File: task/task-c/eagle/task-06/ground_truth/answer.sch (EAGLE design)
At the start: 12 parts, among them IC1 16F84, U1 78L05

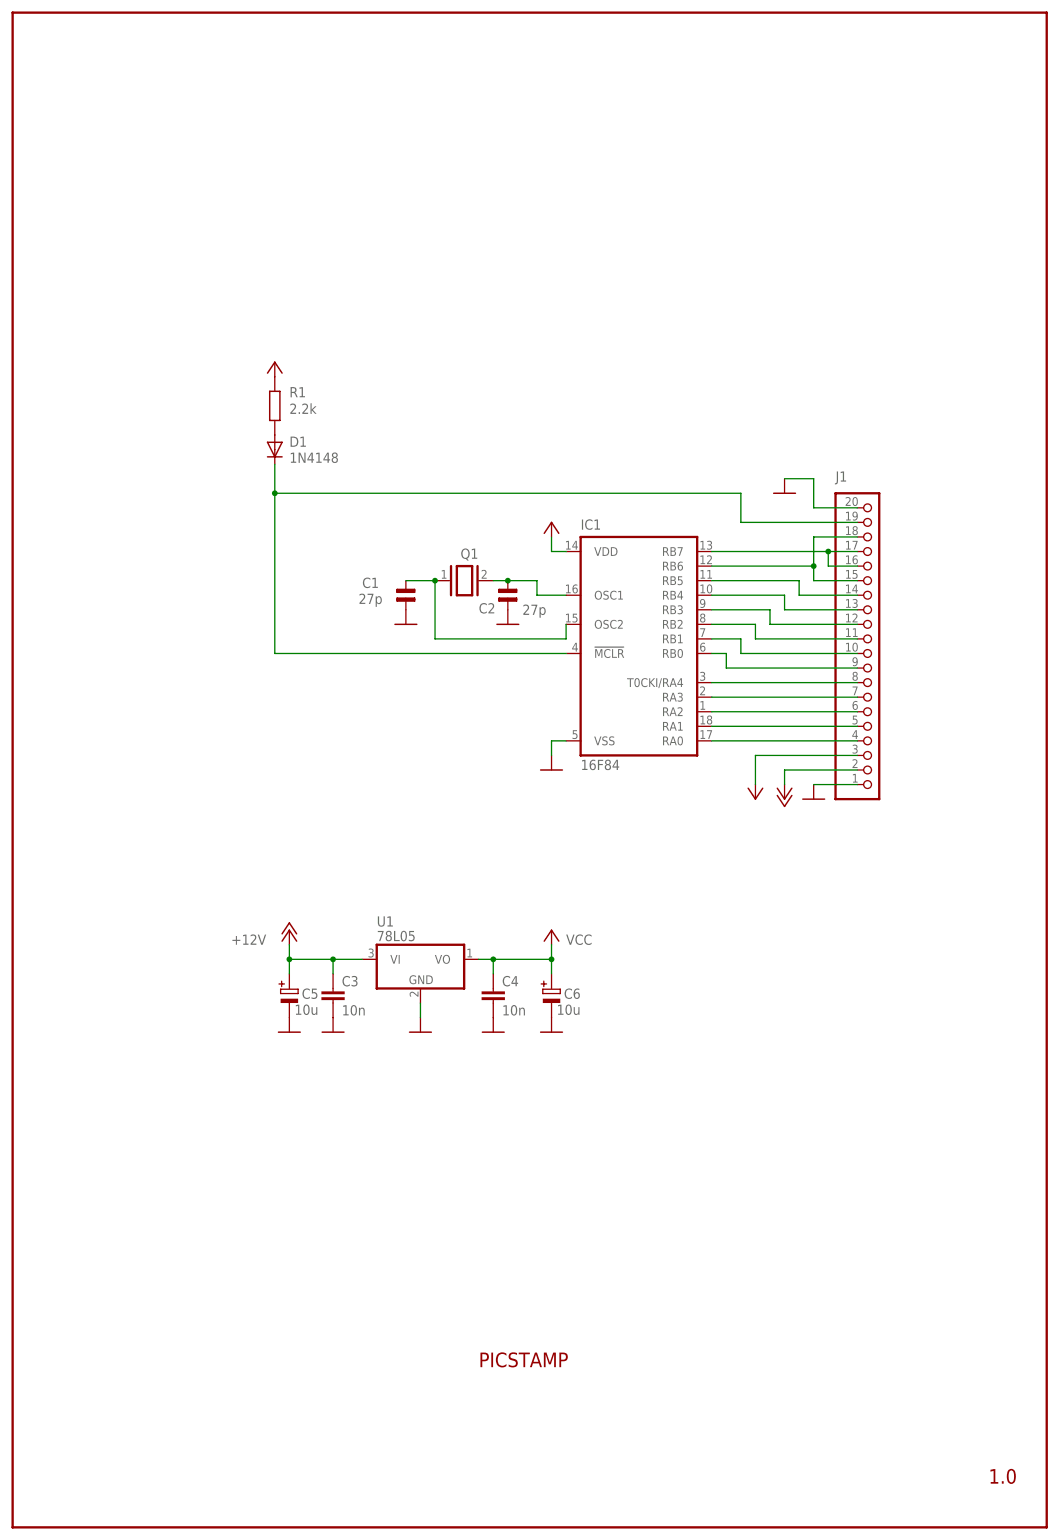
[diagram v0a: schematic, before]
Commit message: Refine engineering task metadata and instructions
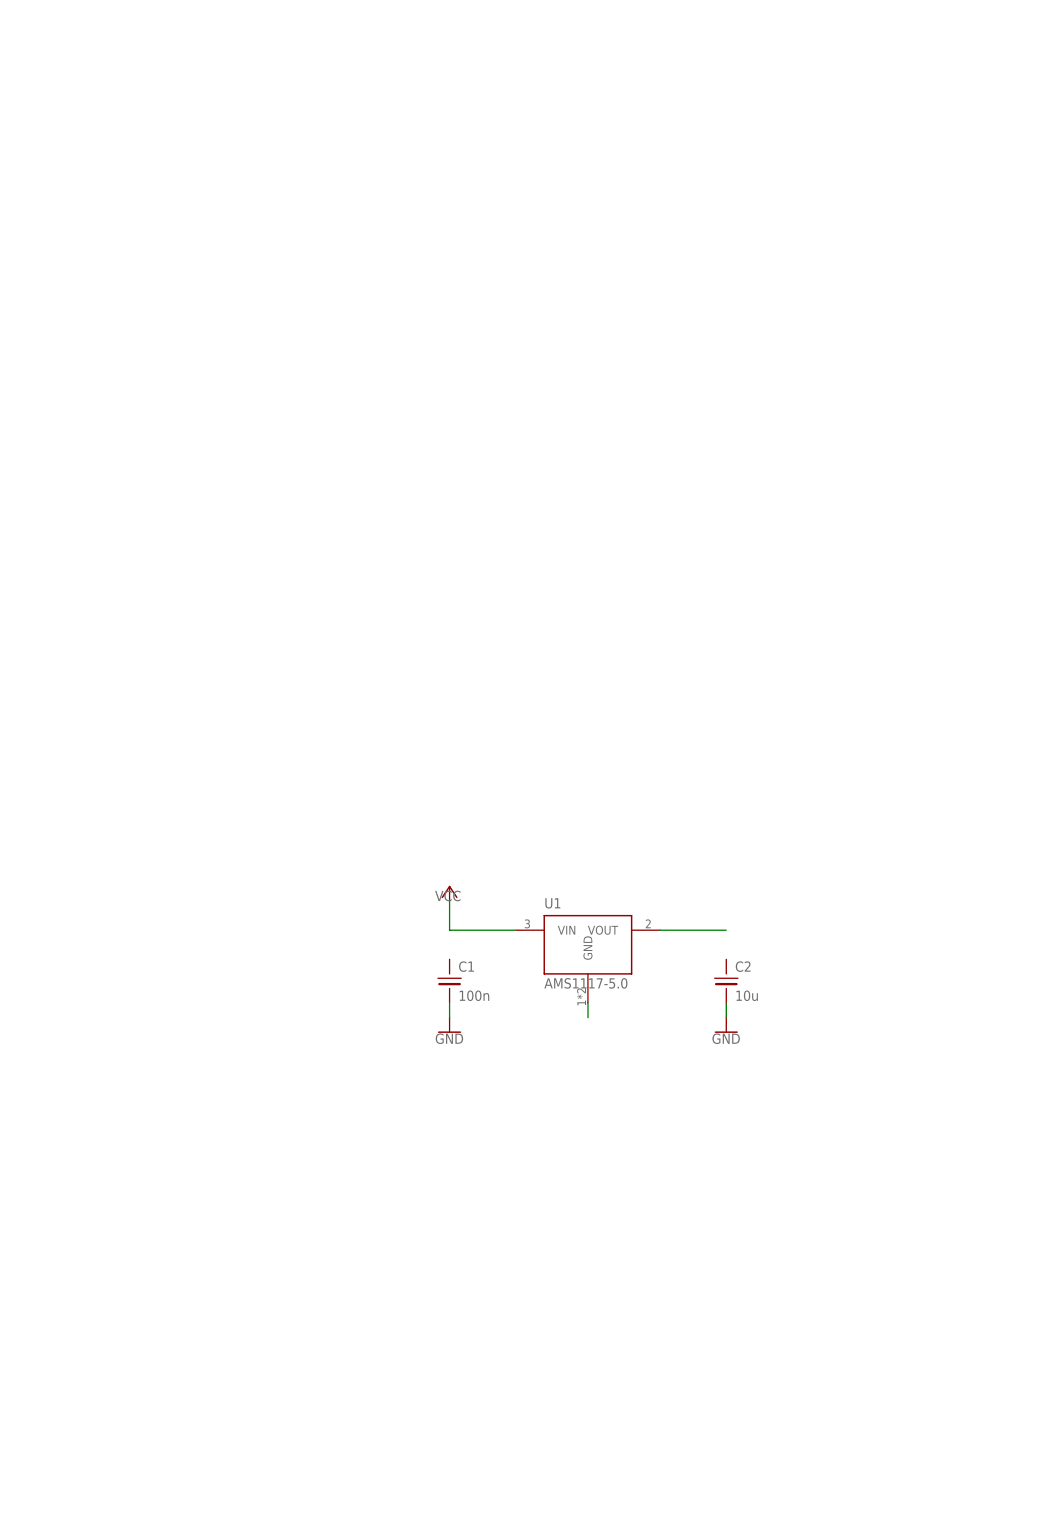
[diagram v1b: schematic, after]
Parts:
- removed C3, C4: 10n, rcl:C-EU025-025X050
- removed C5, C6: 10u, polcap:E2,5-6
- removed D1: 1N4148, diode:1N4148
- removed IC1: 16F84, microchip:PIC16F84AP
- removed J1: (no value), PINHEAD:PINHD-1X20
- removed Q1: (no value), special:XTAL/S
- removed R1: 2.2k, rcl:R-EU_0207/10
- C1: value 27p -> 100n; device capacitor-wima:C2.5/2 -> rcl:C-EU050-025X075
- C2: value 27p -> 10u; device capacitor-wima:C2.5/2 -> rcl:C-EU050-025X075
- U1: value 78L05 -> AMS1117-5.0; device linear:78LXXZ -> v-reg:AMS1117-5.0SOT223
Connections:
- removed net +12V: C3.2, C5.+, J1.2, U1.VI
- removed net A0: IC1.RA0, J1.4
- removed net A1: IC1.RA1, J1.5
- removed net A2: IC1.RA2, J1.6
- removed net A3: IC1.RA3, J1.7
- removed net A4: IC1.T0CKI/RA4, J1.8
- removed net B0: IC1.RB0, J1.9
- removed net B1: IC1.RB1, J1.10
- removed net B2: IC1.RB2, J1.11
- removed net B3: IC1.RB3, J1.12
- removed net B4: IC1.RB4, J1.13
- removed net B5: IC1.RB5, J1.14
- removed net B6: IC1.RB6, J1.15, J1.18
- removed net B7: IC1.RB7, J1.16, J1.17
- removed net N$1: D1.C, IC1.!MCLR, J1.19
- removed net N$2: D1.A, R1.1
- removed net N$3: C2.2, IC1.OSC1, Q1.2
- removed net N$4: C1.2, IC1.OSC2, Q1.1
- removed net VCC: C4.2, C6.+, IC1.VDD, J1.3, R1.2, U1.VO
- new net VIN: C1.1, U1.VIN
- new net VOUT: C2.1, U1.VOUT
- net GND: now also C1.2, C2.2; no longer C1.1, C2.1, C3.1, C4.1, C5.-, C6.-, IC1.VSS, J1.1, J1.20
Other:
- note removed: "1.0"
- note removed: "PICSTAMP"
